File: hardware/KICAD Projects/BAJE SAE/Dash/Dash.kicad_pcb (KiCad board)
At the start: 2 copper layers, 54 x 54 mm, 1 part, among them U1 28-SOIC

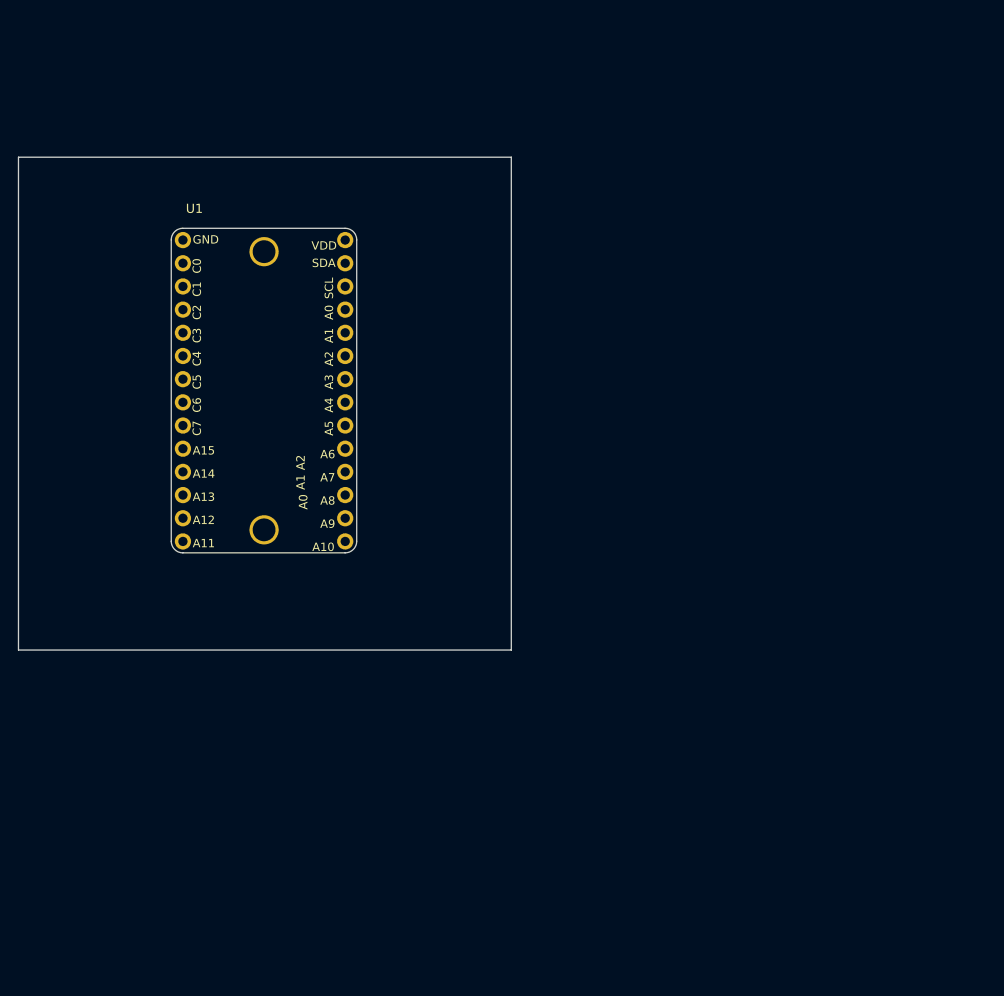
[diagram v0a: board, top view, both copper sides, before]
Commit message: dash <3
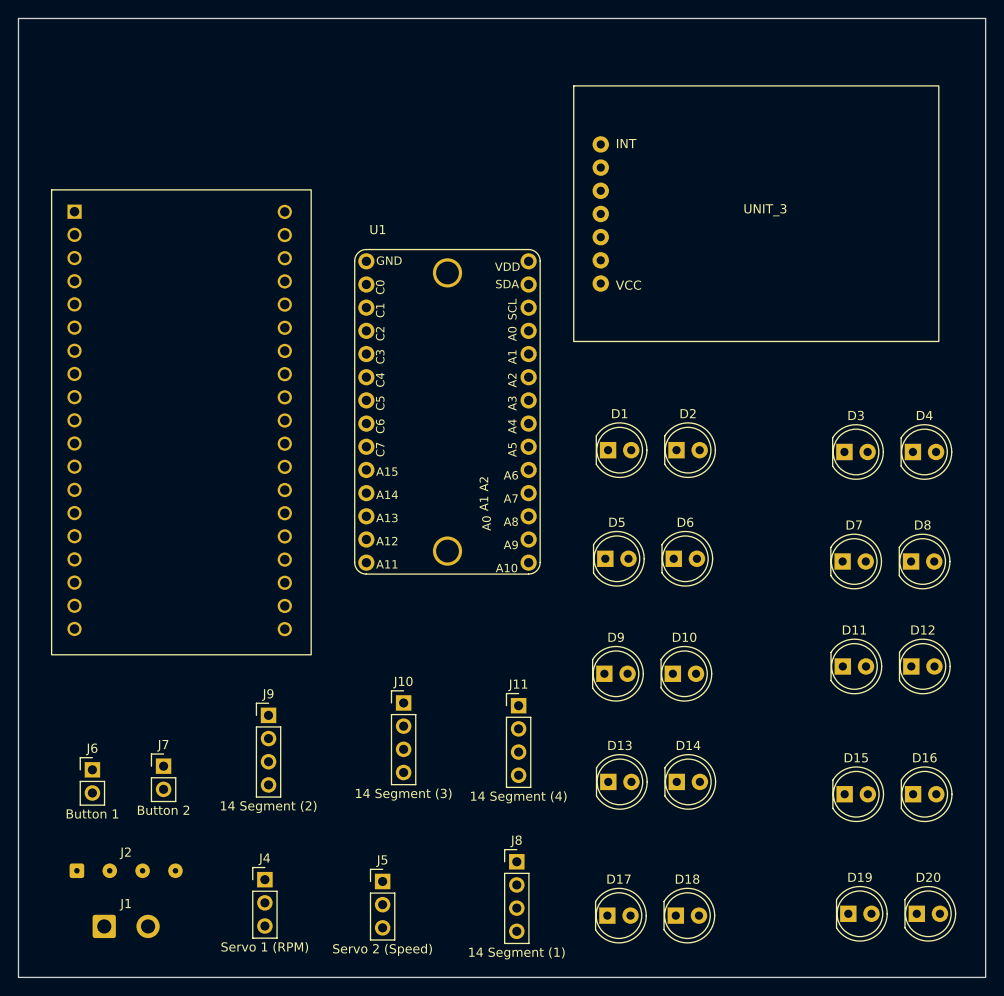
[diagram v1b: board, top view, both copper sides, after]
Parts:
- added D1: LED, LED_THT:LED_D5.0mm, F.Cu at (179.6, 94.7)
- added D10: LED, LED_THT:LED_D5.0mm, F.Cu at (186.7, 119.2)
- added D11: LED, LED_THT:LED_D5.0mm, F.Cu at (205.3, 118.4)
- added D12: LED, LED_THT:LED_D5.0mm, F.Cu at (212.8, 118.4)
- added D13: LED, LED_THT:LED_D5.0mm, F.Cu at (179.6, 131.1)
- added D14: LED, LED_THT:LED_D5.0mm, F.Cu at (187.1, 131.1)
- added D15: LED, LED_THT:LED_D5.0mm, F.Cu at (205.5, 132.4)
- added D16: LED, LED_THT:LED_D5.0mm, F.Cu at (213.0, 132.4)
- added D17: LED, LED_THT:LED_D5.0mm, F.Cu at (179.5, 145.7)
- added D18: LED, LED_THT:LED_D5.0mm, F.Cu at (187.0, 145.7)
- added D19: LED, LED_THT:LED_D5.0mm, F.Cu at (205.9, 145.5)
- added D2: LED, LED_THT:LED_D5.0mm, F.Cu at (187.1, 94.7)
- added D20: LED, LED_THT:LED_D5.0mm, F.Cu at (213.4, 145.5)
- added D3: LED, LED_THT:LED_D5.0mm, F.Cu at (205.5, 94.9)
- added D4: LED, LED_THT:LED_D5.0mm, F.Cu at (213.0, 94.9)
- added D5: LED, LED_THT:LED_D5.0mm, F.Cu at (179.3, 106.6)
- added D6: LED, LED_THT:LED_D5.0mm, F.Cu at (186.8, 106.6)
- added D7: LED, LED_THT:LED_D5.0mm, F.Cu at (205.3, 106.9)
- added D8: LED, LED_THT:LED_D5.0mm, F.Cu at (212.8, 106.9)
- added D9: LED, LED_THT:LED_D5.0mm, F.Cu at (179.2, 119.2)
- added J1: Conn_01x02, Connector_Wire:SolderWire-0.75sqmm_1x02_P4.8mm_D1.25mm_OD2.3mm, F.Cu at (124.4, 146.9)
- added J10: 14 Segment (3), Connector_PinHeader_2.54mm:PinHeader_1x04_P2.54mm_Vertical, F.Cu at (157.2, 122.4)
- added J11: 14 Segment (4), Connector_PinHeader_2.54mm:PinHeader_1x04_P2.54mm_Vertical, F.Cu at (169.8, 122.7)
- added J2: CAN to outer connector, Connector_Wire:SolderWire-0.1sqmm_1x04_P3.6mm_D0.4mm_OD1mm, F.Cu at (121.4, 140.8)
- added J4: Servo 1 (RPM), Connector_PinHeader_2.54mm:PinHeader_1x03_P2.54mm_Vertical, F.Cu at (142.0, 141.8)
- added J5: Servo 2 (Speed), Connector_PinHeader_2.54mm:PinHeader_1x03_P2.54mm_Vertical, F.Cu at (154.9, 142.0)
- added J6: Button 1, Connector_PinHeader_2.54mm:PinHeader_1x02_P2.54mm_Vertical, F.Cu at (123.1, 129.7)
- added J7: Button 2, Connector_PinHeader_2.54mm:PinHeader_1x02_P2.54mm_Vertical, F.Cu at (130.9, 129.3)
- added J8: 14 Segment (1), Connector_PinHeader_2.54mm:PinHeader_1x04_P2.54mm_Vertical, F.Cu at (169.6, 139.8)
- added J9: 14 Segment (2), Connector_PinHeader_2.54mm:PinHeader_1x04_P2.54mm_Vertical, F.Cu at (142.4, 123.8)
- added UNIT_1: ESP32-DEVKITC-32D, BAJA SAE:MODULE_ESP32-DEVKITC-32D, F.Cu at (132.9, 87.5)
- added UNIT_3: CAN Bus, BAJA SAE:HiLetgo CAN Bus (Facing Up), F.Cu at (196.8, 68.8)
- U1: value 28-SOIC -> ~; footprint BAJA SAE:Adafruit HT16K33 breakout -> BAJA SAE:LED Breakout
- moved U1 20.2 mm to (162.1, 71.3)
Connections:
- U1 pad 1: (no net) -> unconnected-(U1-GND-Pad1)
- U1 pad 10: (no net) -> unconnected-(U1-A15-Pad10)
- U1 pad 11: (no net) -> unconnected-(U1-A14-Pad11)
- U1 pad 12: (no net) -> unconnected-(U1-A13-Pad12)
- U1 pad 13: (no net) -> unconnected-(U1-A12-Pad13)
- U1 pad 14: (no net) -> unconnected-(U1-A11-Pad14)
- U1 pad 2: (no net) -> C0
- U1 pad 3: (no net) -> C1
- U1 pad 4: (no net) -> C2
- U1 pad 5: (no net) -> C3
- U1 pad 6: (no net) -> C4
- U1 pad 7: (no net) -> C5
- U1 pad 8: (no net) -> C6
- U1 pad 9: (no net) -> C7
- U1 pad P$1: GND -> (no net)
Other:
- board size 54 x 54 mm -> 106 x 105.1 mm
